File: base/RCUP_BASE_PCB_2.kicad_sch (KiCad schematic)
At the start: 42 parts, among them J1 Conn_01x20_Pin, J2 Conn_01x20_Pin, J3 Conn_01x20_Pin, J4 Conn_01x20_Pin, U3 BNO055

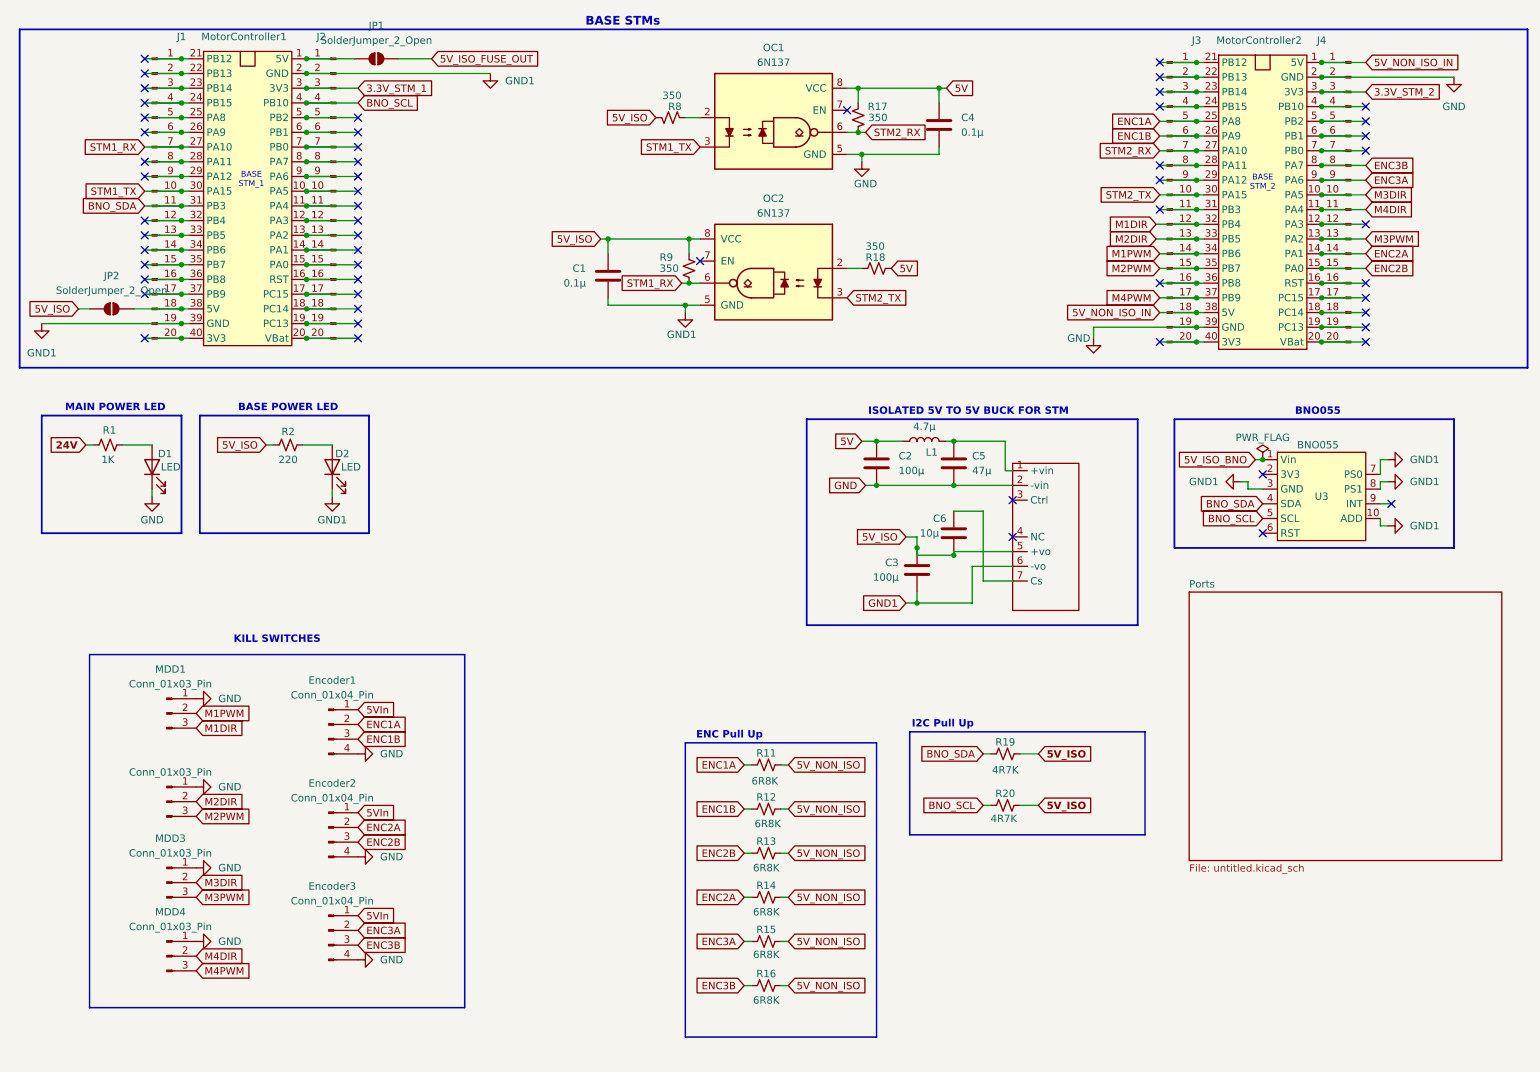
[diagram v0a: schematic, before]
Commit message: fixed all the previous issues added mpu footprint
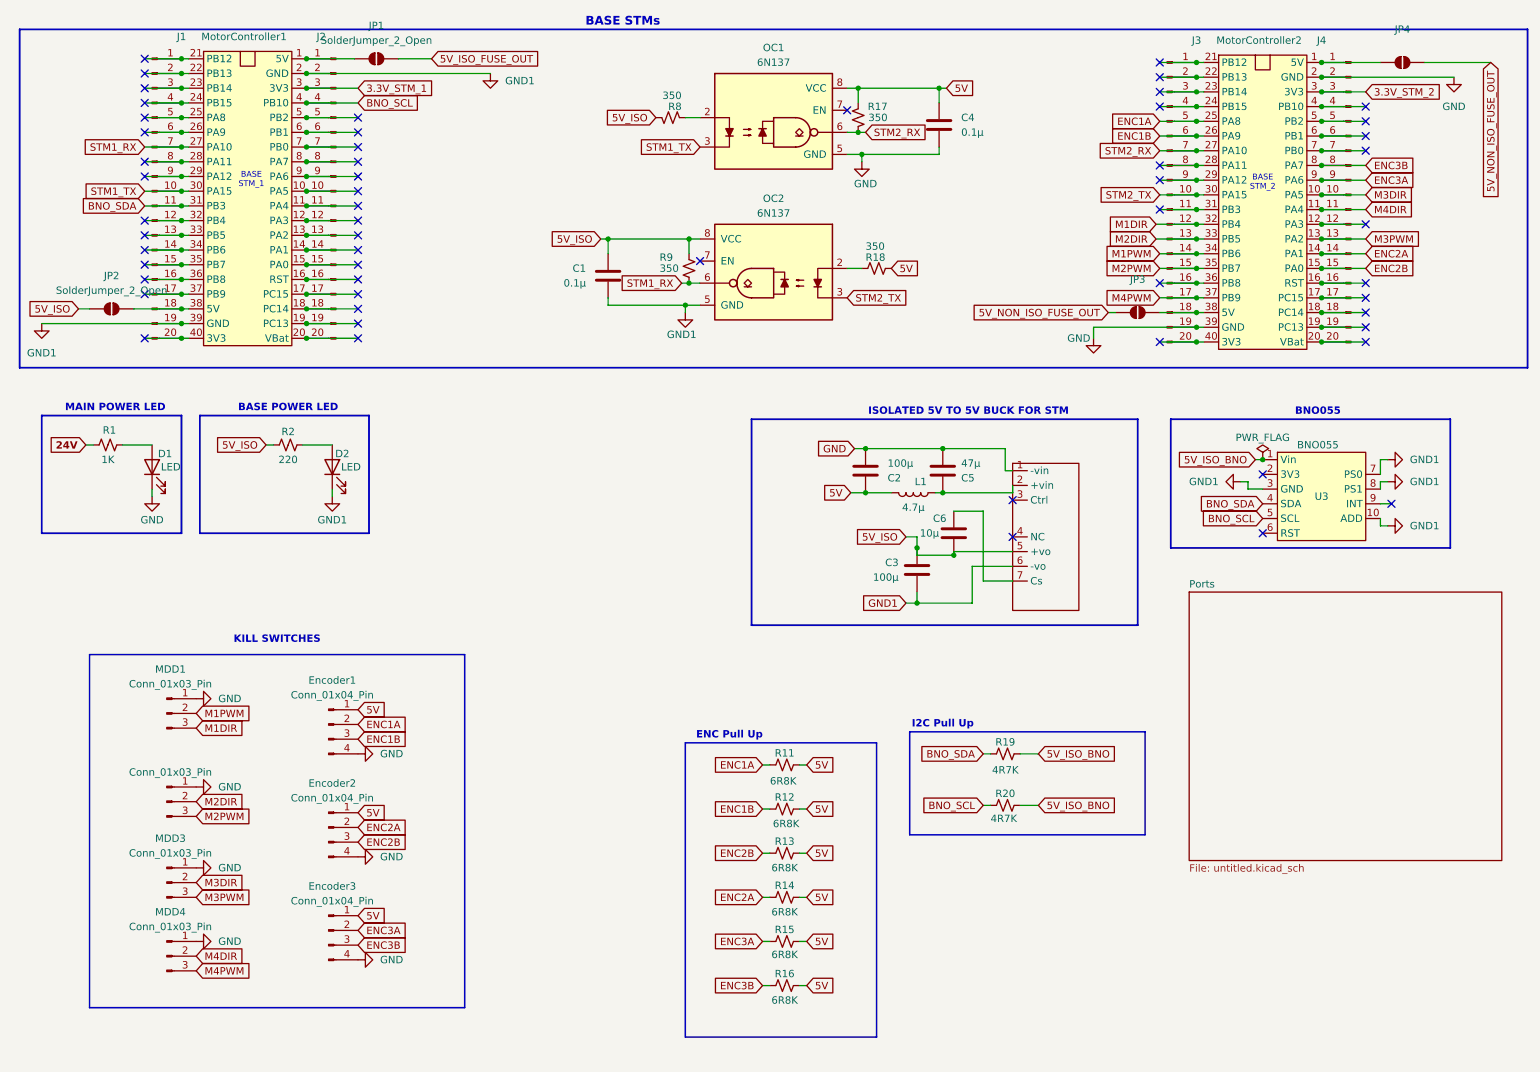
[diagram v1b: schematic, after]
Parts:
- added JP3, JP4: SolderJumper_2_Open, Jumper:SolderJumper-2_P1.3mm_Open_RoundedPad1.0x1.5mm, symbol Jumper:SolderJumper_2_Open
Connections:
- net 5VIn is gone; now on net 5V: Encoder1.1 (Pin_1), Encoder2.1 (Pin_1), Encoder3.1 (Pin_1)
- net 5V_NON_ISO is gone; now on net 5V: R11.2, R12.2, R13.2, R14.2, R15.2, R16.2
- net 5V_ISO: no longer R19.2, R20.2
- net 5V_ISO_BNO: now also R19.2, R20.2
- net GND: now also U2.1 (-vin); no longer U2.2 (-vin)
- net at C5.1, L1.2: now also U2.2 (+vin); no longer U2.1 (+vin)
- net 5V_NON_ISO_IN: no longer names the net of J3.18 (Pin_18), MotorController2.38 (5V)
- net 5V_NON_ISO_IN: now also JP3.2 (B); no longer J4.1 (Pin_1), MotorController2.1 (5V)
- new net: J4.1 (Pin_1), JP4.1 (A), MotorController2.1 (5V)
- new net 5V_NON_ISO_FUSE_OUT: JP3.1 (A), JP4.2 (B)
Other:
- moved on the sheet: C2, C5, L1, R11, R12, R13, R14, R15, R16

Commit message: routing and stm orientation fixed
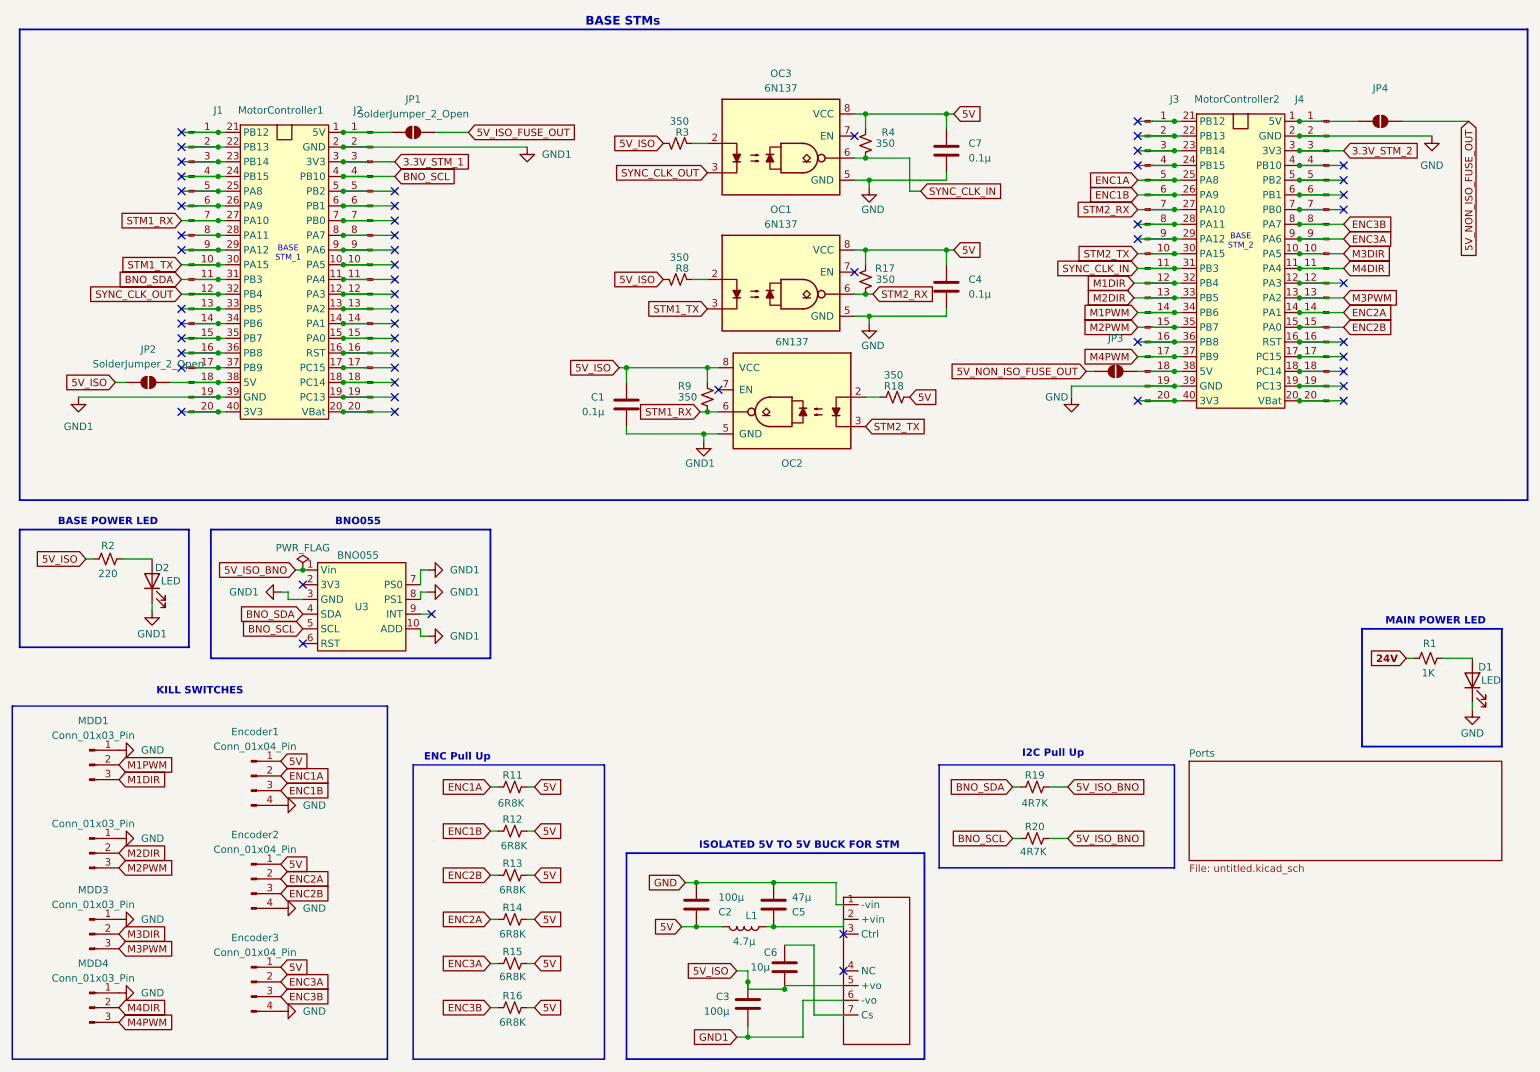
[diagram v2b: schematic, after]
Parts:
- added C7: 0.1µ, Capacitor_SMD:C_0603_1608Metric_Pad1.08x0.95mm_HandSolder, symbol Device:C
- added OC3: 6N137, PCM_Package_DIP_AKL:DIP-8_W7.62mm_LongPads, symbol PCM_Optocoupler_Logic_AKL:6N137
- added R3, R4: 350, PCM_Resistor_SMD_AKL:R_0603_1608Metric_Pad0.98x0.95mm_HandSolder, symbol Device:R_Small_US
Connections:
- net 5V: now also C7.1, OC3.8 (VCC), R4.1
- net 5V_ISO: now also R3.1
- net GND: now also C7.2, OC3.5 (GND)
- net SYNC_CLK_IN: now reaches J3.11 (Pin_11), MotorController2.31 (PB3)
- net SYNC_CLK_IN: now also OC3.6, R4.2
- net SYNC_CLK_OUT: now reaches J1.12 (Pin_12), MotorController1.32 (PB4)
- net SYNC_CLK_OUT: now also OC3.3
- new net: OC3.2, R3.2
- no-connect marks 57 -> 56
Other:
- moved on the sheet: C1, C2, C3, C4, C5, C6, D1, D2, Encoder1, Encoder2, Encoder3, J1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
